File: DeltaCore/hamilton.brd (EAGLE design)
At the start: 40 x 30 mm, 66 parts, among them Q3 MOSFET-NCHANNEL_SOT23-3, Q4 MOSFET-NCHANNEL_SOT23-3, Q5 MOSFET-NCHANNEL_SOT23-3, Q6 MOSFET-NCHANNEL_SOT23-3, Q7 NFET_AON7408, Q8 NFET_AON7408, U1 SAMR21, U10 PCA9557, U2 APDS9007, U3 MMA7660FC, U4 AT30TS74, U5 MCP73871-2AAI/ML, U7 BQ29718, U8 MCP1824ST-3302E/DB, U9 TPS61090, X1 XTAL

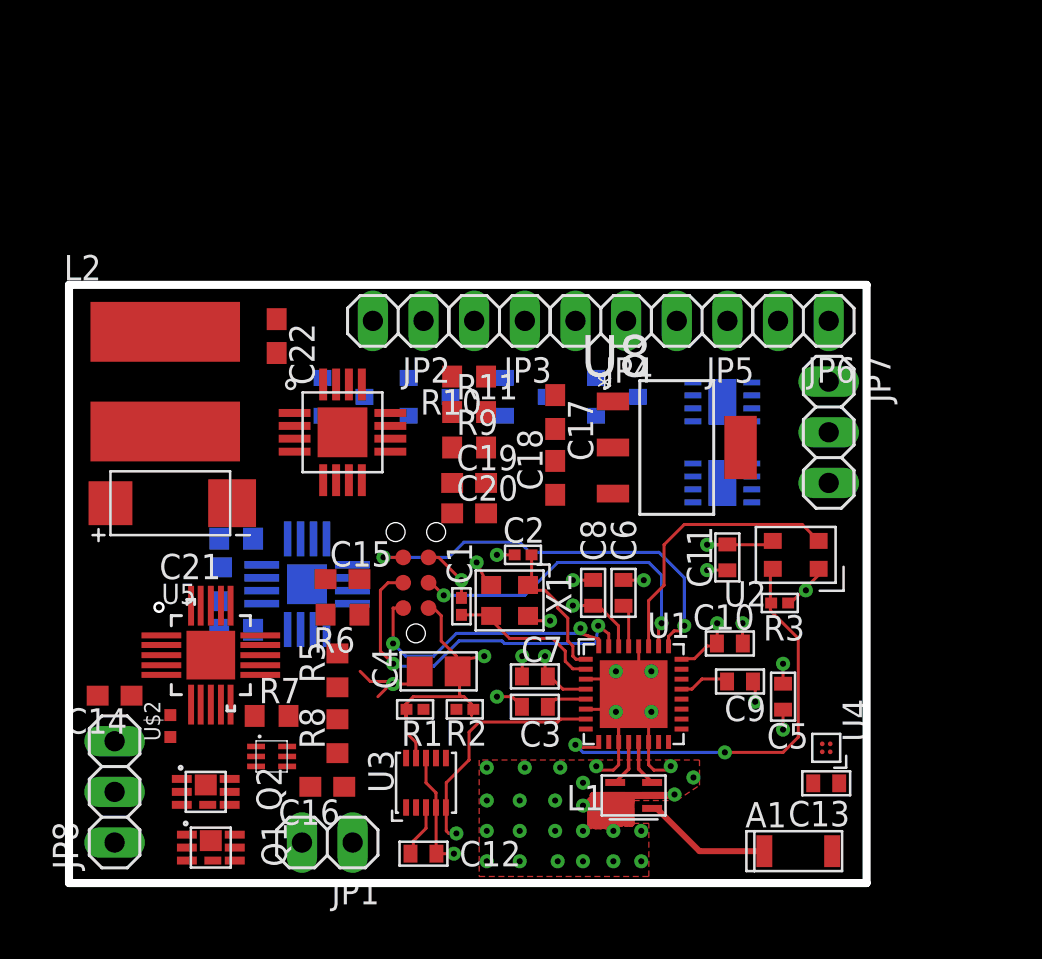
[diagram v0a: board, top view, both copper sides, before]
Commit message: more board
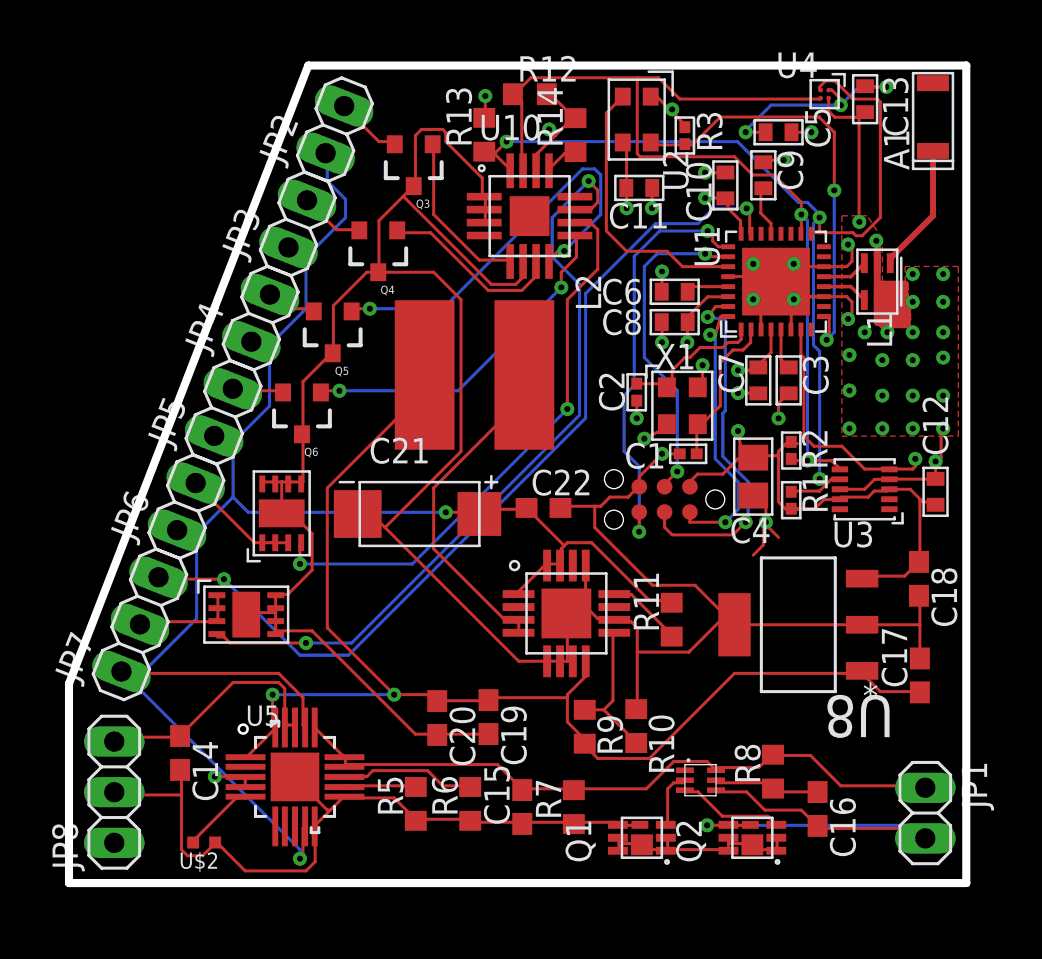
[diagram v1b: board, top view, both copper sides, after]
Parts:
- moved A1 37.4 mm to (43.3, 38.4), turned to 90 degrees
- moved JP7 35.9 mm to (3.56, 13.0), turned to 68.5 degrees
- moved C13 34.4 mm to (39.9, 39.3), turned to 270 degrees
- moved U4 32.8 mm to (37.9, 39.6), turned to 270 degrees
- moved JP6 32.3 mm to (5.89, 18.9), turned to 68.5 degrees
- moved C12 31.4 mm to (43.5, 19.6), turned to 90 degrees
- moved R14 30.1 mm to (25.4, 37.5), flipped to the top, turned to 90 degrees
- moved JP1 30.0 mm to (42.9, 3.51), turned to 270 degrees
- moved R12 29.1 mm to (23.1, 39.6), flipped to the top, turned to 0 degrees
- moved L1 28.5 mm to (40.5, 30.2), turned to 270 degrees
- moved C5 28.3 mm to (35.6, 37.7), turned to 180 degrees
- moved Q2 27.5 mm to (34.3, 2.27), turned to 90 degrees
- moved U3 26.5 mm to (39.9, 19.7), turned to 90 degrees
- moved C9 25.4 mm to (34.8, 35.5), turned to 270 degrees
- moved Q8 24.8 mm to (8.89, 13.5), flipped to the top
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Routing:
- net GND: track 60.5 -> 248.1 mm
- net 5V: track 0.00 -> 97.7 mm, vias 0 -> 3
- net OUT: track 0.00 -> 62.7 mm, vias 0 -> 2
- net SDA: track 0.00 -> 51.4 mm, vias 0 -> 3
- net SCL: track 0.00 -> 50.1 mm, vias 0 -> 2
- net D25: track 0.00 -> 45.4 mm, vias 0 -> 2
- net N$41: track 0.00 -> 38.8 mm, vias 0 -> 2
- net N$20: track 0.00 -> 34.1 mm
- net N$40: track 0.00 -> 28.6 mm, vias 0 -> 2
- net +3V3: track 33.9 -> 60.3 mm, vias 6 -> 10
- net N$25: track 0.00 -> 24.9 mm, vias 0 -> 1
- net N$32: track 0.00 -> 21.2 mm, vias 0 -> 2
- net N$33: track 0.00 -> 17.3 mm, vias 0 -> 2
- net N$27: track 0.00 -> 17.0 mm
- net VCC: track 0.00 -> 12.5 mm
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- added copper zone on layer 15, net +3V3
- added copper zone on layer 2, net GND
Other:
- board size 40 x 30 mm -> 45 x 41 mm
